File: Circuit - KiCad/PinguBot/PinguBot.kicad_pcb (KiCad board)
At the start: 2 copper layers, 136.8 x 150 mm, 26 parts, among them J1 Jack-DC, J2 Conn_01x08_Pin, J3 Conn_01x08_Pin, U1 LM386, U3 LM7805_TO220, U4 TSOP45xx, U5 ESP32_DEVKITC

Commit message: Circuit Improvement
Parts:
- J2, J3: footprint Connector_PinSocket_2.54mm:PinSocket_1x08_P2.54mm_Vertical -> Connector_PinHeader_2.54mm:PinHeader_1x08_P2.54mm_Vertical
- R1: footprint Resistor_THT:R_Axial_DIN0204_L3.6mm_D1.6mm_P7.62mm_Horizontal -> Resistor_THT:R_Axial_DIN0207_L6.3mm_D2.5mm_P10.16mm_Horizontal
- R4: footprint Resistor_THT:R_Axial_DIN0204_L3.6mm_D1.6mm_P7.62mm_Horizontal -> Resistor_THT:R_Axial_DIN0207_L6.3mm_D2.5mm_P7.62mm_Horizontal
- moved DisplayOled1 70.2 mm to (83.8, 100.3), turned to 90 degrees
- moved C2 37.5 mm to (93.3, 129.8), turned to 180 degrees
- moved C1 28.8 mm to (72.4, 152.9)
- moved C3 28.8 mm to (86.3, 167.9)
- moved R1 28.8 mm to (79.6, 156.7)
- moved R2 28.8 mm to (59.5, 137.4)
- moved Speaker1 28.8 mm to (60.1, 152.2)
- moved ServoMotorOne1 24.7 mm to (57.4, 71.7)
- moved ServoMotorTwo1 24.7 mm to (57.8, 89.0)
- moved R4 24.3 mm to (93.3, 135.8), turned to 180 degrees
- moved MotorOne1 24.3 mm to (153.7, 64.7)
- moved MotorTwo1 22.8 mm to (153.6, 75.2)
- moved R3 21.7 mm to (115.2, 146.8)
- moved J1 19.9 mm to (159.2, 154.0), turned to 0 degrees
- moved U1 18.6 mm to (70.7, 139.8), turned to 0 degrees
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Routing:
- net 5V: track 175.5 -> 337.0 mm
- net 3.3V: track 0.00 -> 106.9 mm
- net S_Motor_OUT_2: track 0.00 -> 99.1 mm
- net S_Motor_OUT_1: track 0.00 -> 91.7 mm, vias 0 -> 1
- net Microphone ADC: track 0.00 -> 72.8 mm
- net MO4: track 0.00 -> 46.1 mm
- net SDA_DISPLAY: track 0.00 -> 43.6 mm
- net MO3: track 0.00 -> 38.0 mm
- net SCL_DISPLAY: track 0.00 -> 37.7 mm
- net MO2: track 0.00 -> 29.9 mm
- net MO1: track 0.00 -> 24.0 mm
- net Net-(R4-Pad2): track 37.1 -> 18.4 mm
- net Speaker DAC: track 104.3 -> 87.0 mm
- net STBY: track 0.00 -> 15.0 mm
- net MB2: track 0.00 -> 15.0 mm
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
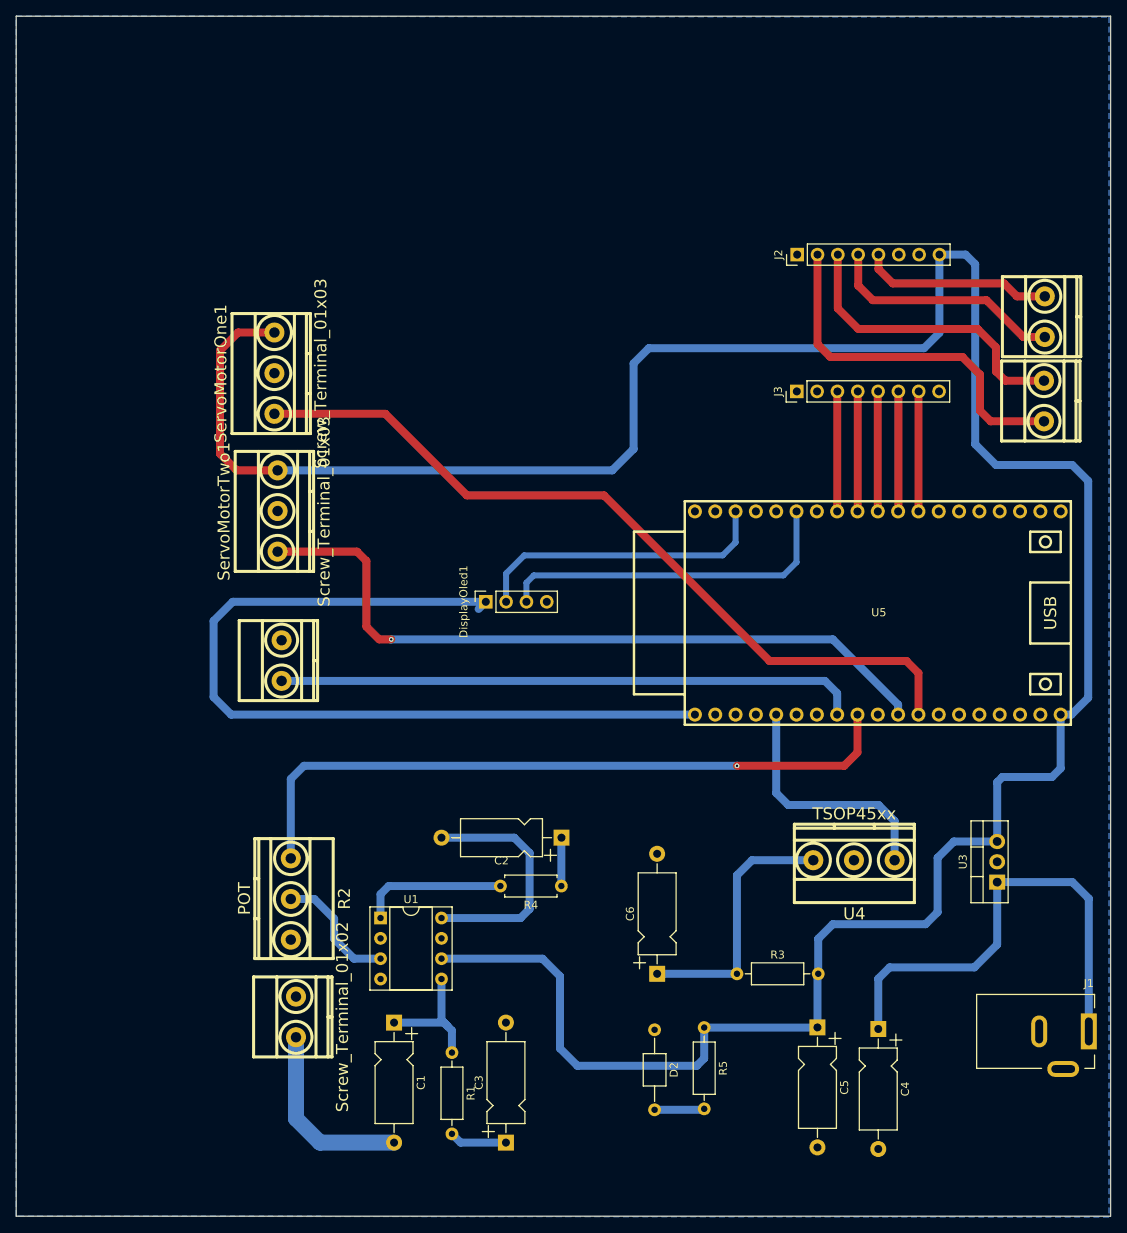
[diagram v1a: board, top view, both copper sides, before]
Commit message: Circuit Improvement | PCB Advanced
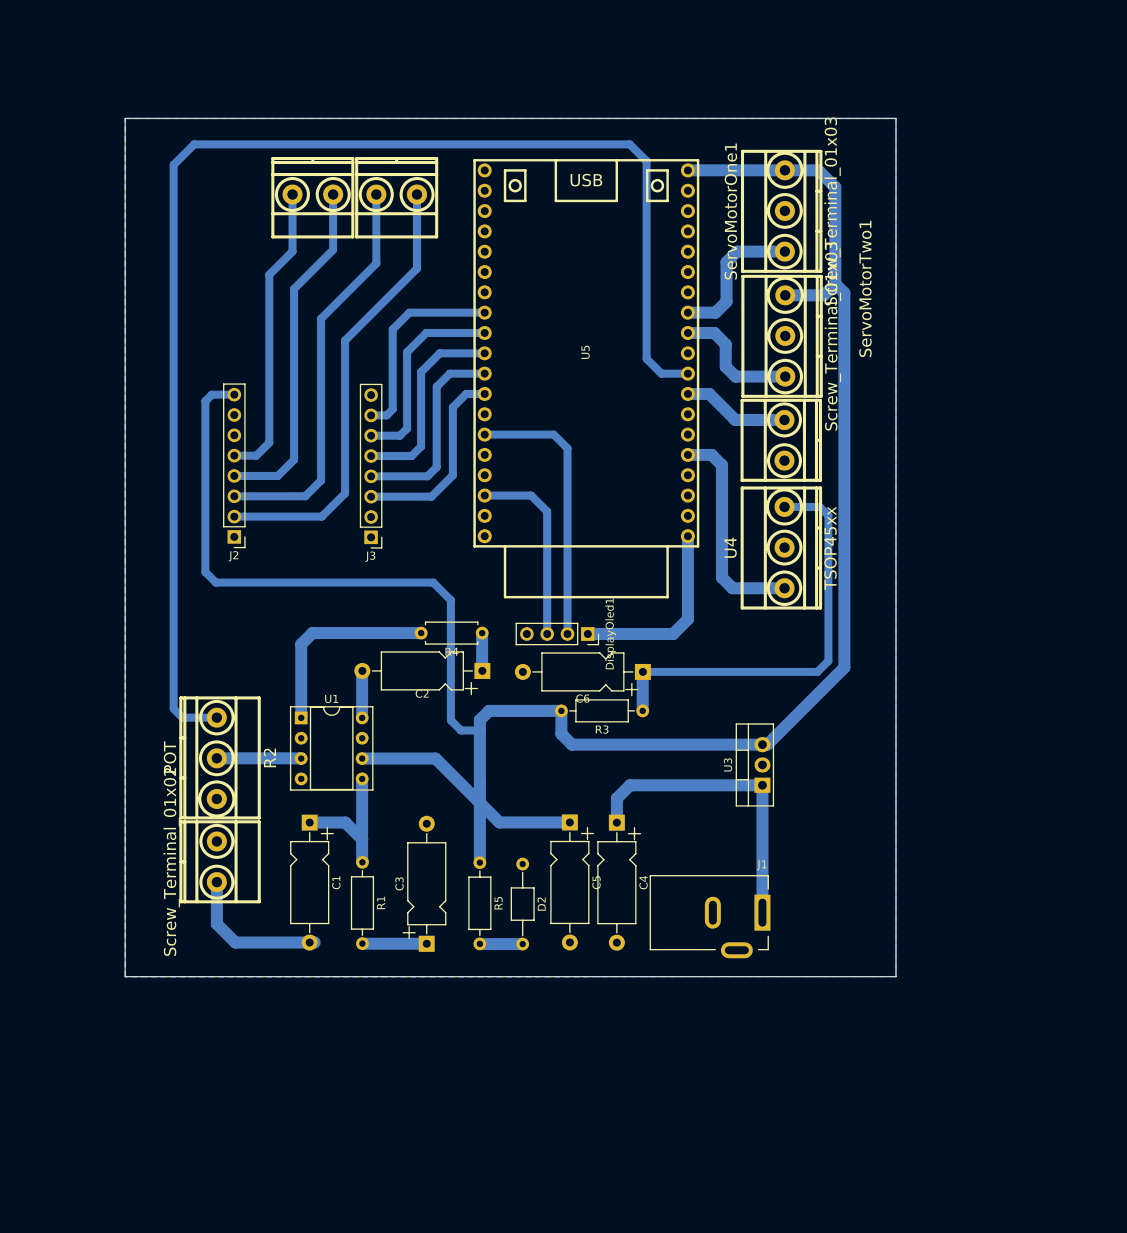
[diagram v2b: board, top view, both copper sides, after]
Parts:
- moved MotorOne1 92.8 mm to (62.2, 49.4), turned to 180 degrees
- moved MotorTwo1 84.9 mm to (72.7, 49.4), turned to 180 degrees
- moved J2 78.7 mm to (52.4, 92.2), turned to 180 degrees
- moved Microphone1 68.6 mm to (121.2, 80.1)
- moved ServoMotorTwo1 67.1 mm to (121.3, 67.1)
- moved ServoMotorOne1 67.0 mm to (121.2, 51.4)
- moved J3 56.2 mm to (69.5, 92.2), turned to 180 degrees
- moved U5 48.8 mm to (96.4, 69.2), turned to 90 degrees
- moved J1 43.4 mm to (118.4, 139.2)
- moved C4 41.6 mm to (100.2, 127.9)
- moved C5 40.2 mm to (94.3, 127.9)
- moved U4 40.0 mm to (121.2, 93.5), turned to 90 degrees
- moved C6 37.8 mm to (103.5, 109.1), turned to 180 degrees
- moved R3 34.9 mm to (103.4, 113.9), turned to 180 degrees
- moved R5 34.8 mm to (83.1, 132.9)
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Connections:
- C1 pad 2: Net-(Speaker1-Pin_1) -> Net-(Speaker1-Pin_2)
- DisplayOled1 pad 2: SCL_DISPLAY -> SDA_DISPLAY
- DisplayOled1 pad 3: SDA_DISPLAY -> SCL_DISPLAY
- Microphone1 pad 1: Microphone ADC -> GND
- Microphone1 pad 2: GND -> Microphone ADC
- Speaker1 pad 1: Net-(Speaker1-Pin_1) -> GND
- Speaker1 pad 2: GND -> Net-(Speaker1-Pin_2)
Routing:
- net 3.3V: track 106.9 -> 23.7 mm
- net S_Motor_OUT_2: track 99.1 -> 18.2 mm
- net Speaker DAC: track 87.0 -> 165.5 mm, vias 1 -> 0
- net S_Motor_OUT_1: track 91.7 -> 16.1 mm, vias 1 -> 0
- net 5V: track 337.0 -> 263.8 mm
- net Microphone ADC: track 72.8 -> 13.4 mm
- net Net-(C2-Pad2): track 30.3 -> 5.88 mm
- net Net-(Speaker1-Pin_1): track 23.7 -> 0.00 mm
- net VIN: track 59.6 -> 37.8 mm
- net Net-(U4-Vs): track 32.6 -> 52.7 mm
- net Net-(Speaker1-Pin_2): track 0.00 -> 17.9 mm
- net SCL_DISPLAY: track 37.7 -> 23.9 mm
- net MO2: track 29.9 -> 43.5 mm
- net MO1: track 24.0 -> 37.3 mm
- net MO3: track 38.0 -> 50.3 mm
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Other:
- board size 136.8 x 150 mm -> 96.3 x 107.3 mm
